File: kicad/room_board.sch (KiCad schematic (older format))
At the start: 20 parts, among them K1 CONN_3, U1 MSP430G2452IN20, U2 7805, U3 DHT

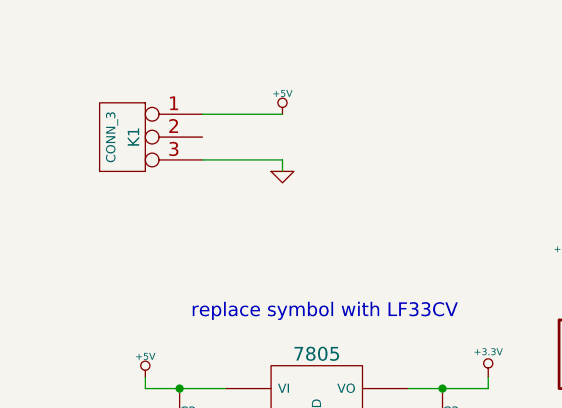
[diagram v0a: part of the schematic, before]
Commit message: update files sent to osh park for board creation
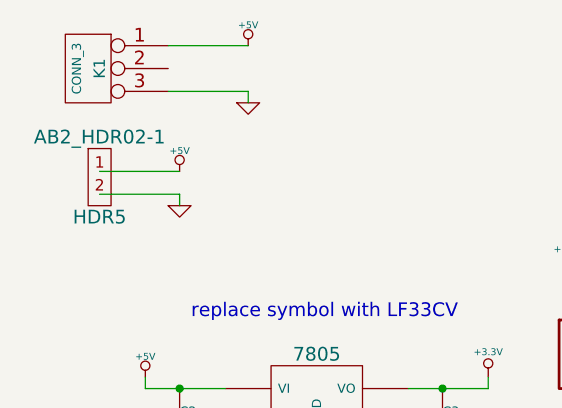
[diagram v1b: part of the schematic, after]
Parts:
- added HDR5: AB2_HDR02-1, symbol AB2_HDR02-1
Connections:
- wire segments 70 -> 73
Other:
- moved on the sheet: K1
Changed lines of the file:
@@
 $EndComp
 $Comp
-L GND #PWR01
+L GND #PWR17
 U 1 1 541A11C0
 P 5400 3300
-F 0 "#PWR01" H 5400 3300 30  0001 C CNN
+F 0 "#PWR17" H 5400 3300 30  0001 C CNN
 F 1 "GND" H 5400 3230 30  0001 C CNN
 F 2 "" H 5400 3300 60  0000 C CNN
@@
 $EndComp
 $Comp
-L GND #PWR02
+L GND #PWR15
 U 1 1 541A11EE
 P 5150 1900
-F 0 "#PWR02" H 5150 1900 30  0001 C CNN
+F 0 "#PWR15" H 5150 1900 30  0001 C CNN
 F 1 "GND" H 5150 1830 30  0001 C CNN
 F 2 "" H 5150 1900 60  0000 C CNN
@@
 $EndComp
 $Comp
-L GND #PWR03
+L GND #PWR4
 U 1 1 541A1DFB
 P 1150 5050
-F 0 "#PWR03" H 1150 5050 30  0001 C CNN
+F 0 "#PWR4" H 1150 5050 30  0001 C CNN
 F 1 "GND" H 1150 4980 30  0001 C CNN
 F 2 "" H 1150 5050 60  0000 C CNN
@@
 $EndComp
 $Comp
-L +5V #PWR04
+L +5V #PWR1
 U 1 1 541A1E6D
 P 1000 2150
-F 0 "#PWR04" H 1000 2240 20  0001 C CNN
+F 0 "#PWR1" H 1000 2240 20  0001 C CNN
 F 1 "+5V" H 1000 2240 30  0000 C CNN
 F 2 "" H 1000 2150 60  0000 C CNN
@@
 $EndComp
 $Comp
-L +3.3V #PWR05
+L +3.3V #PWR8
 U 1 1 541A1FA0
 P 2500 2150
-F 0 "#PWR05" H 2500 2110 30  0001 C CNN
+F 0 "#PWR8" H 2500 2110 30  0001 C CNN
 F 1 "+3.3V" H 2500 2260 30  0000 C CNN
 F 2 "" H 2500 2150 60  0000 C CNN
@@
 $EndComp
 $Comp
-L GND #PWR06
+L GND #PWR7
 U 1 1 541A203B
 P 1750 2650
-F 0 "#PWR06" H 1750 2650 30  0001 C CNN
+F 0 "#PWR7" H 1750 2650 30  0001 C CNN
 F 1 "GND" H 1750 2580 30  0001 C CNN
 F 2 "" H 1750 2650 60  0000 C CNN
@@
 $EndComp
 $Comp
-L GND #PWR07
+L GND #PWR23
 U 1 1 541B579F
 P 7450 1800
-F 0 "#PWR07" H 7450 1800 30  0001 C CNN
+F 0 "#PWR23" H 7450 1800 30  0001 C CNN
 F 1 "GND" H 7450 1730 30  0001 C CNN
 F 2 "" H 7450 1800 60  0000 C CNN
@@
 $EndComp
 $Comp
-L GND #PWR08
+L GND #PWR25
 U 1 1 541B6049
 P 8350 1700
-F 0 "#PWR08" H 8350 1700 30  0001 C CNN
+F 0 "#PWR25" H 8350 1700 30  0001 C CNN
 F 1 "GND" H 8350 1630 30  0001 C CNN
 F 2 "" H 8350 1700 60  0000 C CNN
@@
 $EndComp
 $Comp
-L +3.3V #PWR09
+L +3.3V #PWR9
 U 1 1 541B7B5F
 P 2850 1700
-F 0 "#PWR09" H 2850 1660 30  0001 C CNN
+F 0 "#PWR9" H 2850 1660 30  0001 C CNN
 F 1 "+3.3V" H 2850 1810 30  0000 C CNN
 F 2 "" H 2850 1700 60  0000 C CNN
@@
 $EndComp
 $Comp
-L +3.3V #PWR010
+L +3.3V #PWR16
 U 1 1 541B7D24
 P 5400 1300
-F 0 "#PWR010" H 5400 1260 30  0001 C CNN
+F 0 "#PWR16" H 5400 1260 30  0001 C CNN
 F 1 "+3.3V" H 5400 1410 30  0000 C CNN
 F 2 "" H 5400 1300 60  0000 C CNN
@@
 $EndComp
 $Comp
-L +3.3V #PWR011
+L +3.3V #PWR21
 U 1 1 541B7FD8
 P 7300 950
-F 0 "#PWR011" H 7300 910 30  0001 C CNN
+F 0 "#PWR21" H 7300 910 30  0001 C CNN
 F 1 "+3.3V" H 7300 1060 30  0000 C CNN
 F 2 "" H 7300 950 60  0000 C CNN
@@
 $EndComp
 $Comp
-L +3.3V #PWR012
+L +3.3V #PWR24
 U 1 1 541B803D
 P 8350 1200
-F 0 "#PWR012" H 8350 1160 30  0001 C CNN
+F 0 "#PWR24" H 8350 1160 30  0001 C CNN
 F 1 "+3.3V" H 8350 1310 30  0000 C CNN
 F 2 "" H 8350 1200 60  0000 C CNN
@@
 $EndComp
 $Comp
-L +3.3V #PWR013
+L +3.3V #PWR22
 U 1 1 541B61D1
 P 7450 1400
-F 0 "#PWR013" H 7450 1360 30  0001 C CNN
+F 0 "#PWR22" H 7450 1360 30  0001 C CNN
 F 1 "+3.3V" H 7450 1510 30  0000 C CNN
 F 2 "" H 7450 1400 60  0000 C CNN
@@
 PIR_OUT
 $Comp
-L +5V #PWR014
+L +5V #PWR12
 U 1 1 5425E4B0
 P 3750 850
-F 0 "#PWR014" H 3750 940 20  0001 C CNN
+F 0 "#PWR12" H 3750 940 20  0001 C CNN
 F 1 "+5V" H 3750 940 30  0000 C CNN
 F 2 "" H 3750 850 60  0000 C CNN
@@
 $EndComp
 $Comp
-L GND #PWR015
+L GND #PWR13
 U 1 1 5425E54A
 P 3750 1100
-F 0 "#PWR015" H 3750 1100 30  0001 C CNN
+F 0 "#PWR13" H 3750 1100 30  0001 C CNN
 F 1 "GND" H 3750 1030 30  0001 C CNN
 F 2 "" H 3750 1100 60  0000 C CNN
@@
 $EndComp
 $Comp
-L GND #PWR016
+L GND #PWR27
 U 1 1 5425FC92
 P 9950 4400
-F 0 "#PWR016" H 9950 4400 30  0001 C CNN
+F 0 "#PWR27" H 9950 4400 30  0001 C CNN
 F 1 "GND" H 9950 4330 30  0001 C CNN
 F 2 "" H 9950 4400 60  0000 C CNN
@@
 $EndComp
 $Comp
-L +3.3V #PWR017
+L +3.3V #PWR26
 U 1 1 5425FE92
 P 9950 3250
-F 0 "#PWR017" H 9950 3210 30  0001 C CNN
+F 0 "#PWR26" H 9950 3210 30  0001 C CNN
 F 1 "+3.3V" H 9950 3360 30  0000 C CNN
 F 2 "" H 9950 3250 60  0000 C CNN
@@
 $EndComp
 $Comp
-L GND #PWR018
+L GND #PWR10
 U 1 1 54261CF5
 P 2850 2950
-F 0 "#PWR018" H 2850 2950 30  0001 C CNN
+F 0 "#PWR10" H 2850 2950 30  0001 C CNN
 F 1 "GND" H 2850 2880 30  0001 C CNN
 F 2 "" H 2850 2950 60  0000 C CNN
@@
 	1150 3800 1850 3800
 $Comp
-L GND #PWR019
+L GND #PWR6
 U 1 1 542639D4
-P 1600 1250
-F 0 "#PWR019" H 1600 1250 30  0001 C CNN
-F 1 "GND" H 1600 1180 30  0001 C CNN
-F 2 "" H 1600 1250 60  0000 C CNN
-F 3 "" H 1600 1250 60  0000 C CNN
-	1    1600 1250
-	1    0    0    -1
-$EndComp
-$Comp
-L +5V #PWR020
+P 1450 950
+F 0 "#PWR6" H 1450 950 30  0001 C CNN
+F 1 "GND" H 1450 880 30  0001 C CNN
+F 2 "" H 1450 950 60  0000 C CNN
+F 3 "" H 1450 950 60  0000 C CNN
+	1    1450 950
+	1    0    0    -1
+$EndComp
+$Comp
+L +5V #PWR5
 U 1 1 54263A4F
-P 1600 1000
-F 0 "#PWR020" H 1600 1090 20  0001 C CNN
-F 1 "+5V" H 1600 1090 30  0000 C CNN
-F 2 "" H 1600 1000 60  0000 C CNN
-F 3 "" H 1600 1000 60  0000 C CNN
-	1    1600 1000
-	1    0    0    -1
-$EndComp
-Wire Wire Line
-	1250 1200 1600 1200
-Wire Wire Line
-	1600 1200 1600 1250
-Wire Wire Line
-	1600 1000 1250 1000
+P 1450 700
+F 0 "#PWR5" H 1450 790 20  0001 C CNN
+F 1 "+5V" H 1450 790 30  0000 C CNN
+F 2 "" H 1450 700 60  0000 C CNN
+F 3 "" H 1450 700 60  0000 C CNN
+	1    1450 700
+	1    0    0    -1
+$EndComp
+Wire Wire Line
+	1100 900  1450 900
+Wire Wire Line
+	1450 900  1450 950
+Wire Wire Line
+	1450 700  1100 700
 $Comp
 L AB2_HDR04-2 HDR2
@@
 	3900 4700 4250 4700
 $Comp
-L GND #PWR021
+L GND #PWR11
 U 1 1 54264903
 P 3350 4450
-F 0 "#PWR021" H 3350 4450 30  0001 C CNN
+F 0 "#PWR11" H 3350 4450 30  0001 C CNN
 F 1 "GND" H 3350 4380 30  0001 C CNN
 F 2 "" H 3350 4450 60  0000 C CNN
@@
 $EndComp
 $Comp
-L +3.3V #PWR022
+L +3.3V #PWR14
 U 1 1 54264C23
 P 4250 4400
-F 0 "#PWR022" H 4250 4360 30  0001 C CNN
+F 0 "#PWR14" H 4250 4360 30  0001 C CNN
 F 1 "+3.3V" H 4250 4510 30  0000 C CNN
 F 2 "" H 4250 4400 60  0000 C CNN
@@
 TX
 $Comp
-L GND #PWR023
+L GND #PWR18
 U 1 1 5426577D
 P 5550 4550
-F 0 "#PWR023" H 5550 4550 30  0001 C CNN
+F 0 "#PWR18" H 5550 4550 30  0001 C CNN
 F 1 "GND" H 5550 4480 30  0001 C CNN
 F 2 "" H 5550 4550 60  0000 C CNN
@@
 RST
 $Comp
-L GND #PWR024
+L GND #PWR20
 U 1 1 54266071
 P 6450 4550
-F 0 "#PWR024" H 6450 4550 30  0001 C CNN
+F 0 "#PWR20" H 6450 4550 30  0001 C CNN
 F 1 "GND" H 6450 4480 30  0001 C CNN
 F 2 "" H 6450 4550 60  0000 C CNN
@@
 $EndComp
 $Comp
-L +3.3V #PWR025
+L +3.3V #PWR19
 U 1 1 54266462
 P 6250 3750
-F 0 "#PWR025" H 6250 3710 30  0001 C CNN
+F 0 "#PWR19" H 6250 3710 30  0001 C CNN
 F 1 "+3.3V" H 6250 3860 30  0000 C CNN
 F 2 "" H 6250 3750 60  0000 C CNN
@@
 L CONN_3 K1
 U 1 1 5429D710
-P 900 1100
-F 0 "K1" V 850 1100 50  0000 C CNN
-F 1 "CONN_3" V 950 1100 40  0000 C CNN
-F 2 "ab2_power:AB2_PB_2MM_JACK_PTH" H 900 1100 60  0001 C CNN
-F 3 "" H 900 1100 60  0000 C CNN
-	1    900  1100
+P 750 800
+F 0 "K1" V 700 800 50  0000 C CNN
+F 1 "CONN_3" V 800 800 40  0000 C CNN
+F 2 "ab2_power:AB2_PB_2MM_JACK_PTH" H 750 800 60  0001 C CNN
+F 3 "" H 750 800 60  0000 C CNN
+	1    750  800
 	-1   0    0    -1
 $EndComp
+$Comp
+L AB2_HDR02-1 HDR5
+U 1 1 543063E2
+P 800 1250
+F 0 "HDR5" H 800 1050 60  0000 C CNN
+F 1 "AB2_HDR02-1" H 800 1400 60  0000 C CNN
+F 2 "" H 800 1250 60  0000 C CNN
+F 3 "" H 800 1250 60  0000 C CNN
+	1    800  1250
+	1    0    0    -1
+$EndComp
+$Comp
+L GND #PWR3
+U 1 1 54306686
+P 1150 1400
+F 0 "#PWR3" H 1150 1400 30  0001 C CNN
+F 1 "GND" H 1150 1330 30  0001 C CNN
+F 2 "" H 1150 1400 60  0000 C CNN
+F 3 "" H 1150 1400 60  0000 C CNN
+	1    1150 1400
+	1    0    0    -1
+$EndComp
+$Comp
+L +5V #PWR2
+U 1 1 5430668C
+P 1150 1250
+F 0 "#PWR2" H 1150 1340 20  0001 C CNN
+F 1 "+5V" H 1150 1340 30  0000 C CNN
+F 2 "" H 1150 1250 60  0000 C CNN
+F 3 "" H 1150 1250 60  0000 C CNN
+	1    1150 1250
+	1    0    0    -1
+$EndComp
+Wire Wire Line
+	800  1350 1150 1350
+Wire Wire Line
+	1150 1350 1150 1400
+Wire Wire Line
+	1150 1250 800  1250
 $EndSCHEMATC
